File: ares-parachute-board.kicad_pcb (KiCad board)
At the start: 2 copper layers, 57 x 88 mm, 181 parts, among them J1 Conn_01x16_Female, J3 Conn_01x02_Male, J4 Conn_ARM_JTAG_SWD_10, J5 Conn_01x03_Pin, J6 MPT 0.5/2-2.54, U1 XC6206P332MR, U2 AP2552W6-7, U3 SR05-ES, U4 W25Q128JVSIQTR, U5 LIS2DW12TR, U6 STM32F103CBTx, U7 LIS2DW12TR, X1 CSTNE8M00G520000R0, X2 Q13FC1350000400

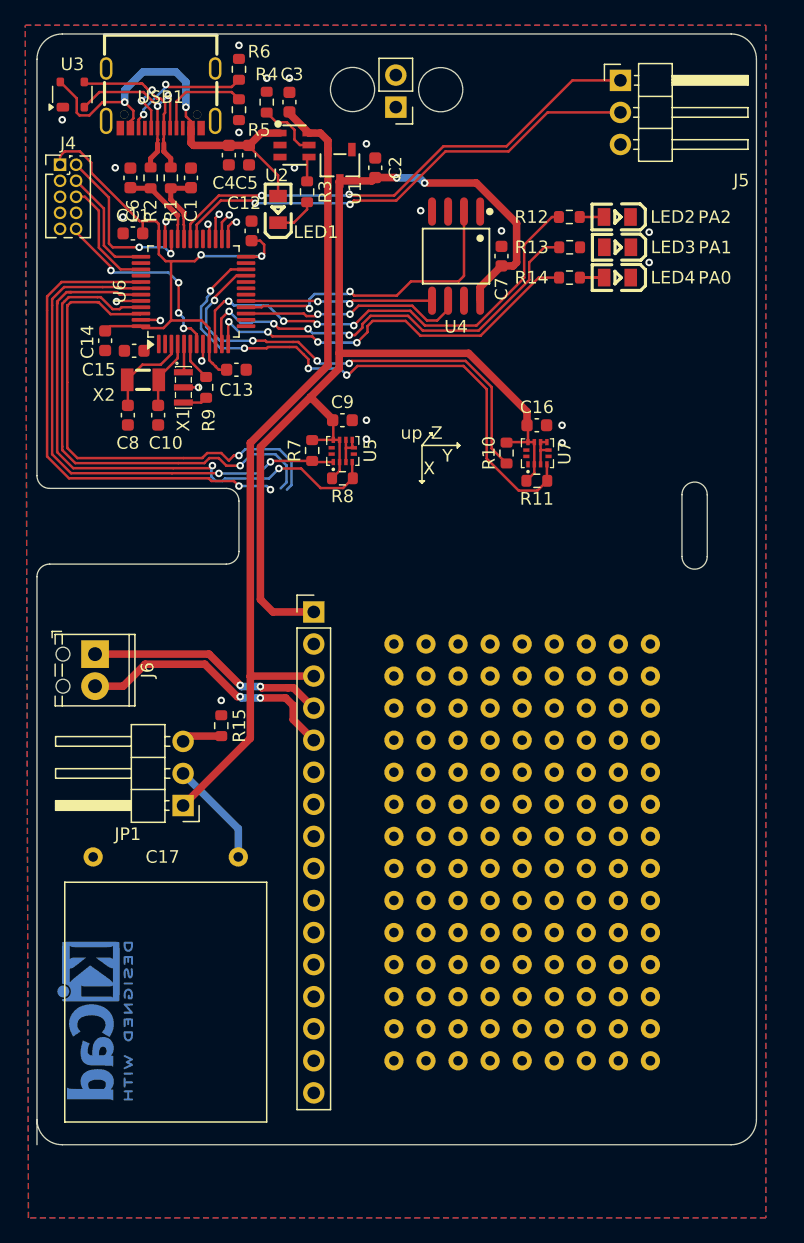
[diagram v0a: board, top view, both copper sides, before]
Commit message: layout done
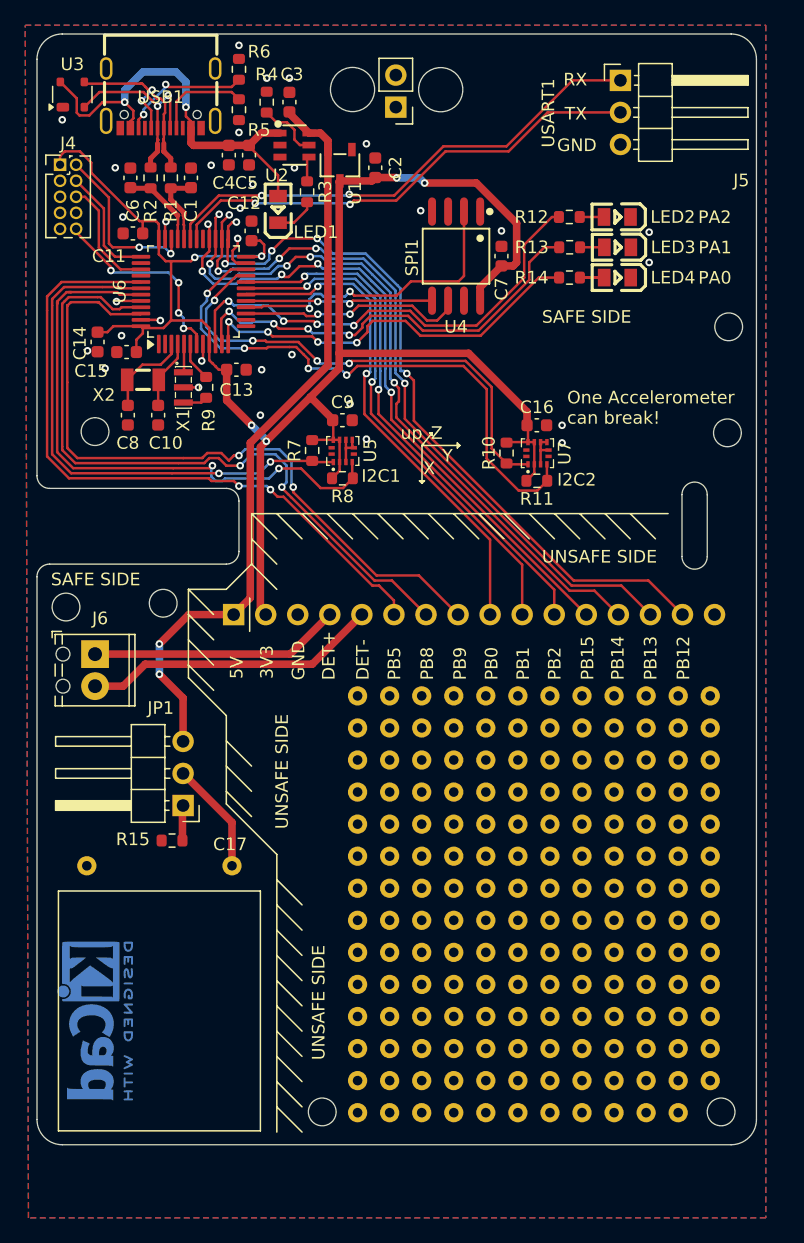
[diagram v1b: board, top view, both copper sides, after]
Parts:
- removed the   at (228.6, 133.3)
- added  : , asyd-parachute:my_pin, F.Cu at (205.4, 124.8)
- added  : , asyd-parachute:my_pin, F.Cu at (207.9, 129.8)
- added  : , asyd-parachute:my_pin, F.Cu at (207.9, 132.4)
- added  : , asyd-parachute:my_pin, F.Cu at (205.4, 112.1)
- added  : , asyd-parachute:my_pin, F.Cu at (210.5, 127.3)
- added  : , asyd-parachute:my_pin, F.Cu at (207.9, 117.1)
- added  : , asyd-parachute:my_pin, F.Cu at (207.9, 119.7)
- added  : , asyd-parachute:my_pin, F.Cu at (205.4, 109.5)
- added  : , asyd-parachute:my_pin, F.Cu at (207.9, 109.5)
- added  : , asyd-parachute:my_pin, F.Cu at (210.5, 119.7)
- added  : , asyd-parachute:my_pin, F.Cu at (207.9, 137.5)
- added  : , asyd-parachute:my_pin, F.Cu at (205.4, 122.2)
- added  : , asyd-parachute:my_pin, F.Cu at (207.9, 112.1)
- added  : , asyd-parachute:my_pin, F.Cu at (210.5, 117.1)
- added  : , asyd-parachute:my_pin, F.Cu at (210.5, 114.6)
- added  : , asyd-parachute:my_pin, F.Cu at (205.4, 129.8)
- added  : , asyd-parachute:my_pin, F.Cu at (205.4, 127.3)
- added  : , asyd-parachute:my_pin, F.Cu at (210.5, 122.2)
- added  : , asyd-parachute:my_pin, F.Cu at (210.5, 132.4)
- added  : , asyd-parachute:my_pin, F.Cu at (210.5, 107.0)
- added  : , asyd-parachute:my_pin, F.Cu at (205.4, 107.0)
- added  : , asyd-parachute:my_pin, F.Cu at (210.5, 109.5)
- added  : , asyd-parachute:my_pin, F.Cu at (210.5, 124.8)
- added  : , asyd-parachute:my_pin, F.Cu at (205.4, 134.9)
- added  : , asyd-parachute:my_pin, F.Cu at (210.5, 104.4)
- added  : , asyd-parachute:my_pin, F.Cu at (205.4, 114.6)
- added  : , asyd-parachute:my_pin, F.Cu at (207.9, 122.2)
- added  : , asyd-parachute:my_pin, F.Cu at (205.4, 119.7)
- added  : , asyd-parachute:my_pin, F.Cu at (207.9, 124.8)
- added  : , asyd-parachute:my_pin, F.Cu at (210.5, 137.5)
- added  : , asyd-parachute:my_pin, F.Cu at (205.4, 104.4)
- added  : , asyd-parachute:my_pin, F.Cu at (205.4, 132.4)
- added  : , asyd-parachute:my_pin, F.Cu at (210.5, 129.8)
- added  : , asyd-parachute:my_pin, F.Cu at (205.4, 117.1)
- added  : , asyd-parachute:my_pin, F.Cu at (207.9, 107.0)
- added  : , asyd-parachute:my_pin, F.Cu at (210.5, 112.1)
- added  : , asyd-parachute:my_pin, F.Cu at (205.4, 137.5)
- added  : , asyd-parachute:my_pin, F.Cu at (207.9, 104.4)
- added  : , asyd-parachute:my_pin, F.Cu at (207.9, 134.9)
- added  : , asyd-parachute:my_pin, F.Cu at (207.9, 114.6)
- added  : , asyd-parachute:my_pin, F.Cu at (210.5, 134.9)
- added  : , asyd-parachute:my_pin, F.Cu at (207.9, 127.3)
- added REF**: MountingHole_2.2mm_M2, MountingHole:MountingHole_2.2mm_M2, F.Cu at (182.3, 97.4)
- added REF**: MountingHole_2.2mm_M2, MountingHole:MountingHole_2.2mm_M2, F.Cu at (234.8, 75.2)
- added REF**: MountingHole_2.2mm_M2, MountingHole:MountingHole_2.2mm_M2, F.Cu at (234.2, 137.4)
- added REF**: MountingHole_2.2mm_M2, MountingHole:MountingHole_2.2mm_M2, F.Cu at (190.0, 97.1)
- added REF**: MountingHole_2.2mm_M2, MountingHole:MountingHole_2.2mm_M2, F.Cu at (234.7, 83.6)
- added REF**: MountingHole_2.2mm_M2, MountingHole:MountingHole_2.2mm_M2, F.Cu at (184.6, 83.5)
- added REF**: MountingHole_2.2mm_M2, MountingHole:MountingHole_2.2mm_M2, F.Cu at (202.6, 137.4)
- moved R15 9.90 mm to (190.7, 115.9), turned to 0 degrees
- moved J1 6.35 mm to (195.6, 98.0), turned to 90 degrees
- moved   6.27 mm to (225.7, 134.9)
- moved   6.27 mm to (225.7, 137.5)
- moved   6.27 mm to (225.7, 109.5)
- moved   6.27 mm to (225.7, 114.6)
- moved   6.27 mm to (225.7, 117.1)
- moved   6.27 mm to (225.7, 104.4)
- moved   6.27 mm to (225.7, 119.7)
- moved   6.27 mm to (225.7, 122.2)
- moved   6.27 mm to (225.7, 127.3)
- moved   6.27 mm to (225.7, 107.0)
- moved   6.27 mm to (225.7, 112.1)
- moved   6.27 mm to (225.7, 124.8)
- moved   6.27 mm to (225.7, 129.8)
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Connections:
- J1 pad 1: +3.3V -> +5V
- J1 pad 10: /PB8 -> /PB1
- J1 pad 11: /PB9 -> /PB2
- J1 pad 12: /PB12 -> /PB15
- J1 pad 13: /PB13 -> /PB14
- J1 pad 14: /PB14 -> /PB13
- J1 pad 15: /PB15 -> /PB12
- J1 pad 16: /PA3 -> unconnected-(J1-Pin_16-Pad16)
- J1 pad 2: GND -> +3.3V
- J1 pad 3: +5V -> GND
- J1 pad 6: /PB0 -> /PB5
- J1 pad 7: /PB1 -> /PB8
- J1 pad 8: /PB2 -> /PB9
- J1 pad 9: /PB5 -> /PB0
- JP1 pad 1: +5V -> Net-(JP1-A)
- JP1 pad 3: Net-(JP1-B) -> +5V
- R15 pad 2: Net-(JP1-B) -> Net-(JP1-A)
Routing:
- net /PB12: track 1.78 -> 59.2 mm, vias 1 -> 5
- net /PB13: track 2.15 -> 57.4 mm, vias 1 -> 5
- net /PB14: track 2.07 -> 55.7 mm, vias 1 -> 5
- net /PB15: track 1.21 -> 52.8 mm, vias 1 -> 5
- net /PB2: track 0.00 -> 42.7 mm, vias 0 -> 2
- net /PB1: track 0.00 -> 41.3 mm, vias 0 -> 2
- net /PB0: track 0.00 -> 40.0 mm, vias 0 -> 2
- net /PB9: track 39.4 -> 56.5 mm, vias 1 -> 2
- net /PB8: track 39.9 -> 55.4 mm, vias 1 -> 2
- net /PB5: track 39.4 -> 53.9 mm
- net +5V: track 66.5 -> 60.0 mm, vias 0 -> 2
- net +3.3V: track 143.1 -> 149.5 mm, vias 4 -> 6
- net Net-(JP1-B): track 3.20 -> 0.00 mm
- net GND: track 13.6 -> 16.6 mm, vias 23 -> 32
- net Net-(JP1-A): track 0.00 -> 2.80 mm
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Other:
- outline, holes or cut-outs redrawn
- board text added: "3V3"
- board text added: "5V"
- board text added: "DET+"
- board text added: "DET-"
- board text added: "GND"
- board text added: "I2C1"
- board text added: "I2C2"
- board text added: "One Accelerometer can break!"
- board text added: "PB0"
- board text added: "PB1"
- board text added: "PB12"
- board text added: "PB13"
- board text added: "PB14"
- board text added: "PB15"
- board text added: "PB2"
- board text added: "PB5"
- board text added: "PB8"
- board text added: "PB9"
- board text added: "RX"
- board text added: "SAFE SIDE"
- board text added: "SPI1"
- board text added: "TX"
- board text added: "UNSAFE SIDE"
- board text added: "USART1"
